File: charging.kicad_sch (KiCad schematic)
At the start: 14 parts, among them J5 S2B-PH-SM4-TB, U2 BQ24075RGT

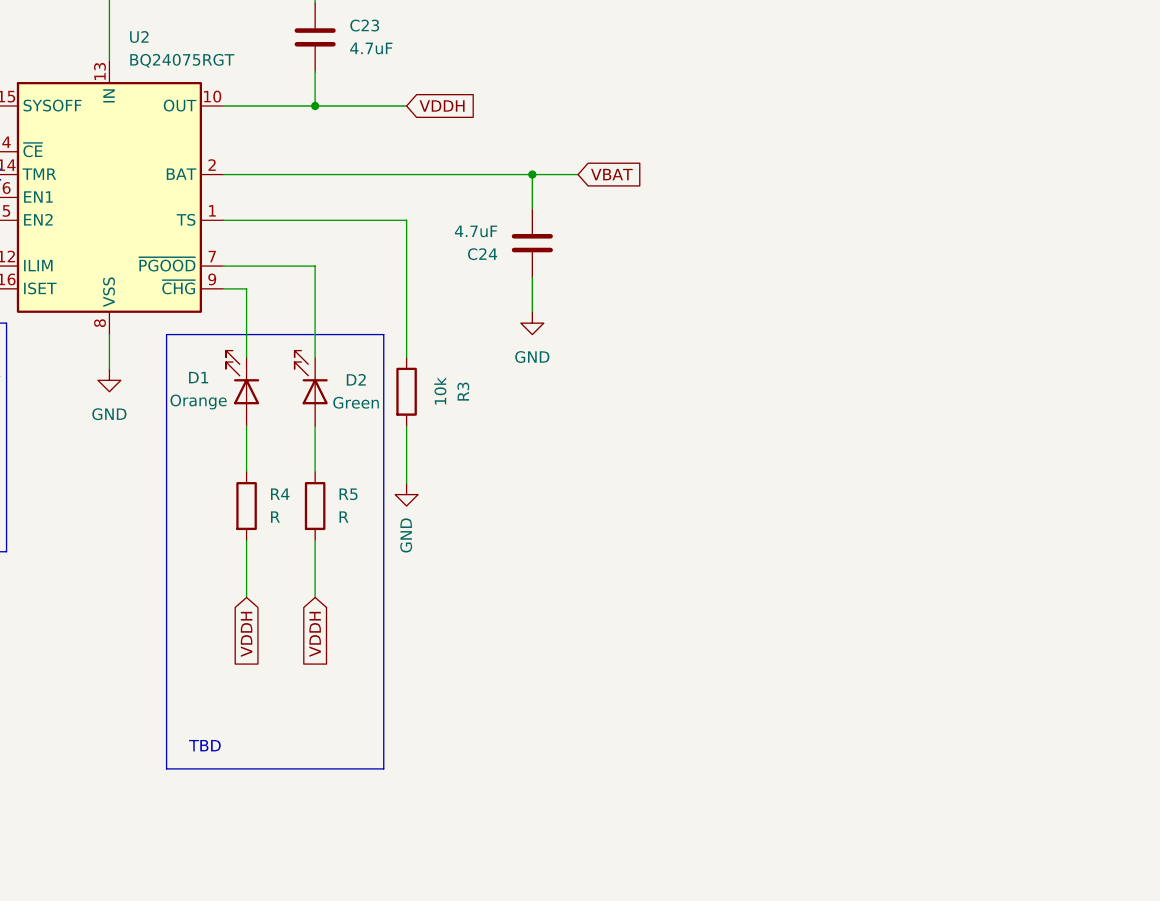
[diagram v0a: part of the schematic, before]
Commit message: Started PCB design
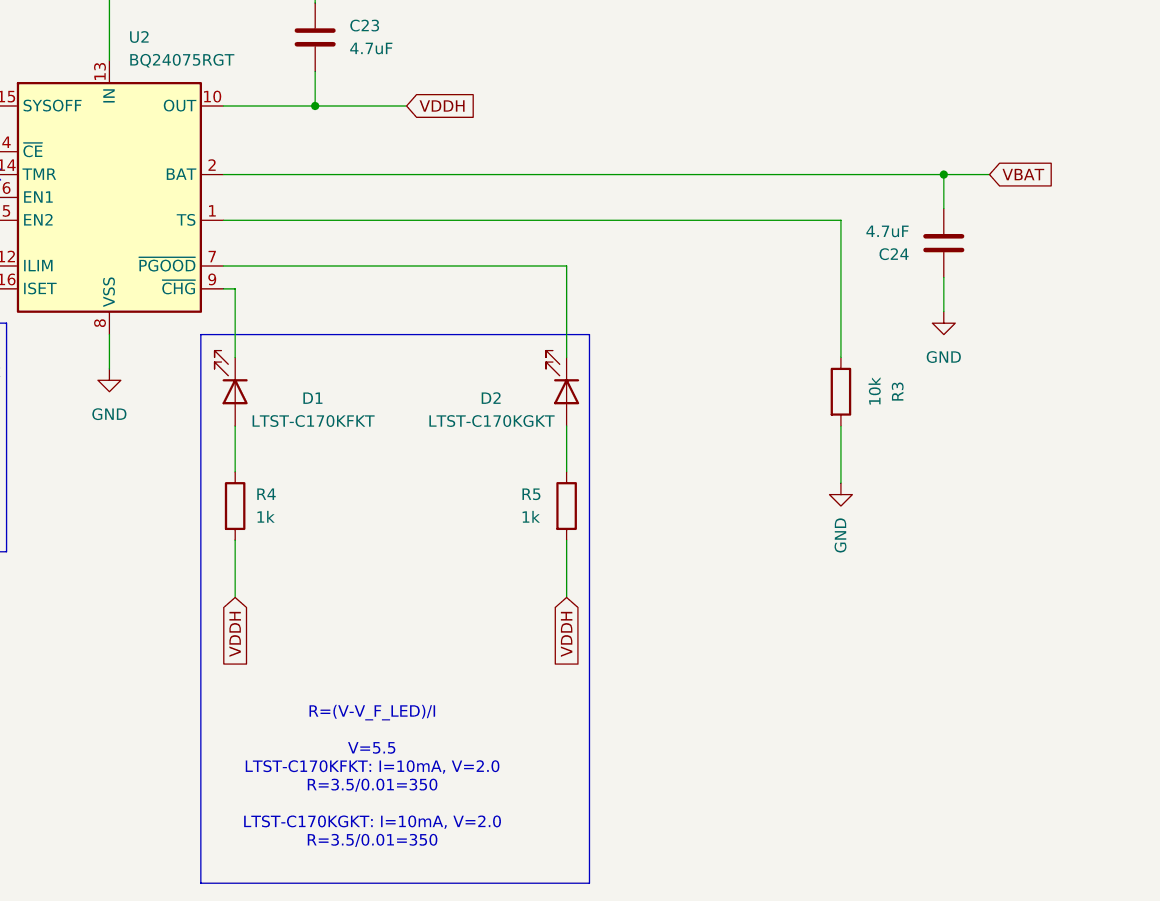
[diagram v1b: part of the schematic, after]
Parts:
- D1: value Orange -> LTST-C170KFKT
- D2: value Green -> LTST-C170KGKT
- R4, R5: value R -> 1k
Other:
- note added: "R=(V-V_F_LED)/I V=5.5 LTST-C170KFKT: I=10mA, V=2.0 R=3.5/0.01=350 LTST-C170KGKT: I=10mA, V=2.0 R=3.5/0.01=350"
- note removed: "TBD"
- moved on the sheet: C24, D1, D2, R3, R4, R5
